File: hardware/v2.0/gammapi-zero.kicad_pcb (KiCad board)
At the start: 4 copper layers, 65 x 30 mm, 209 parts, among them IC1 IS42S16160J-6BLI, IC3 LM4040AIM3-2.0_NOPB, IC4 LTC2622IMS8#PBF, IC5 LTC6409IUDB#TRPBF, IC6 ADS6122IRHBT, J1 Conn_02x20_Counter_Clockwise, J2 GPDI_C_1.3, J3 USB_C_Receptacle_USB2.0_14P, J4 USB_C_Receptacle_USB2.0_14P, J5 USB_C_Receptacle_USB2.0_14P, J6 Micro_SD_Card_Det2, J7 RSP-122811-01, J8 BM04B-ACHSS-A-GAN-TF_LF__SN_, SW1 SW_Push, SW2 SW_Push, U1 ECP5U-25F-CABGA256, U10 TPD2EUSB30A, U12 W25Q128JVS, U2 LTC3407AEDD-2_PBF, U3 TLV62569DBV, U5 TCR5FM18A, U6 PCA9306DC1, U7 TPD2EUSB30A, U8 TPD2EUSB30A, U9 FT231XQ, Y1 SG-8018CG 50.000000MHz, Y2 SG-8018CG 50.000000MHz

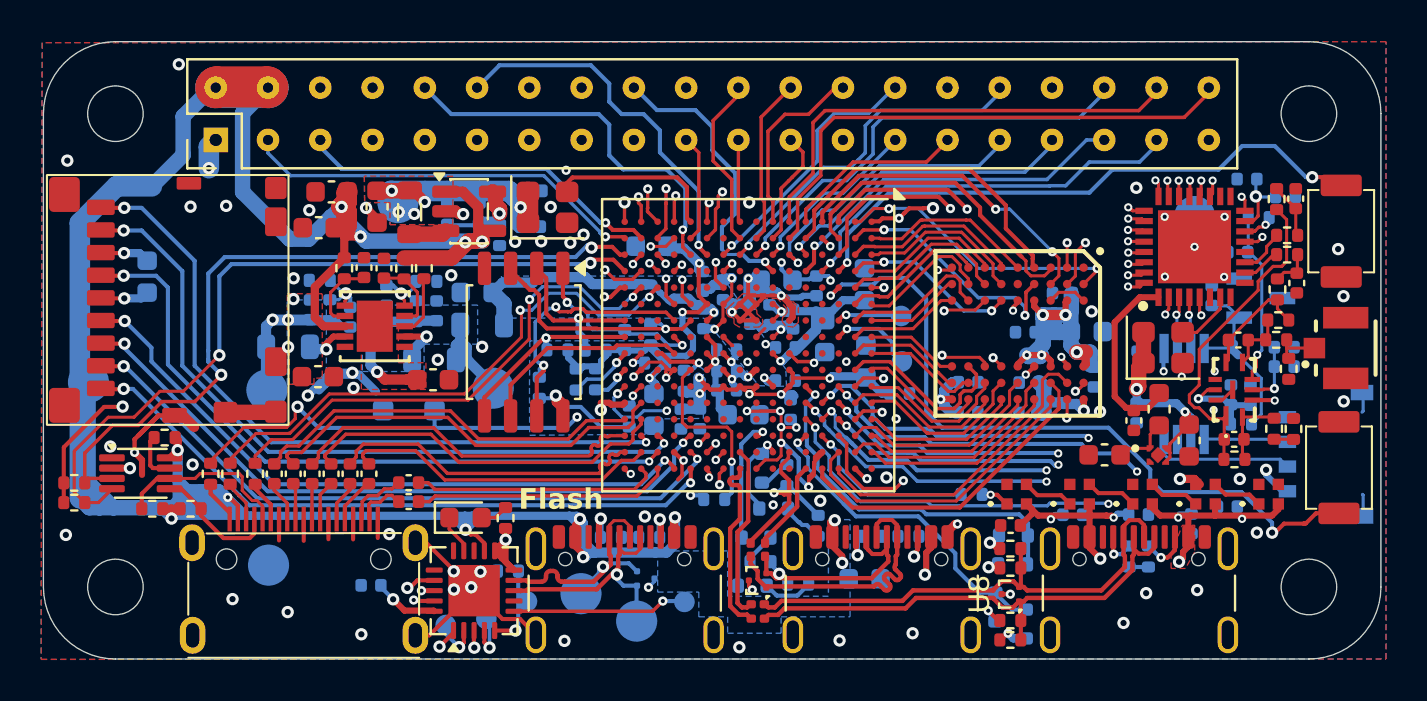
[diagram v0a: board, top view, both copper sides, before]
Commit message: Layout fixes
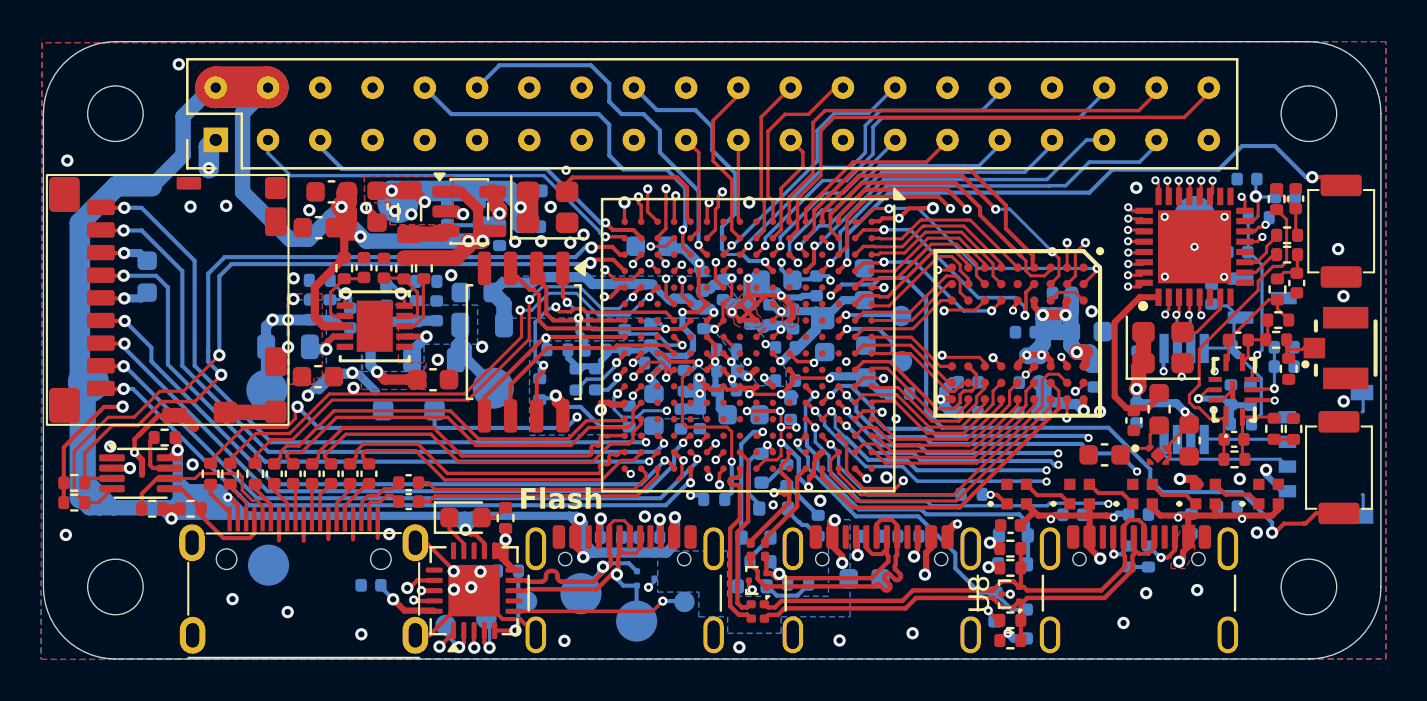
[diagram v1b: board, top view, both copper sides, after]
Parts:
- moved R47 0.07 mm to (139.9, 106.9)
- moved C83 0.07 mm to (172.5, 102.3)
- moved IC3 0.07 mm to (175.0, 102.5)

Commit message: Layout adjustments
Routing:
- net +3V3: track 144.3 -> 143.7 mm
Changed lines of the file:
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@@
 	)
 	(segment
-		(start 144.97153 108.71153)
-		(end 145.351296 108.71153)
+		(start 144.400001 107.760001)
+		(end 145.351296 108.711296)
 		(width 0.2)
 		(layer "In2.Cu")
@@
 	)
 	(segment
-		(start 146.125 117.65)
-		(end 146.044024 117.65)
+		(start 149.775 115.782247)
+		(end 148.891247 116.666)
 		(width 0.2)
 		(layer "In2.Cu")
@@
 	)
 	(segment
-		(start 137.204322 118.909)
-		(end 136.46591 118.909)
+		(start 137.402589 118.907411)
+		(end 137.205911 118.907411)
 		(width 0.2)
 		(layer "In2.Cu")
@@
 	)
 	(segment
-		(start 144.400001 107.209964)
-		(end 144.400001 108.140001)
+		(start 145.351296 108.71153)
+		(end 145.380765 108.741)
 		(width 0.2)
 		(layer "In2.Cu")
@@
 	)
 	(segment
-		(start 141.316 116.941)
-		(end 138.435667 116.941)
+		(start 148.618024 109.059)
+		(end 148.891 109.331976)
 		(width 0.2)
 		(layer "In2.Cu")
@@
 	)
 	(segment
-		(start 145.367171 117.65)
-		(end 142.025 117.65)
+		(start 145.351296 108.711296)
+		(end 145.351296 108.71153)
 		(width 0.2)
 		(layer "In2.Cu")
@@
 	)
 	(segment
-		(start 145.351296 108.71153)
-		(end 145.380765 108.741)
+		(start 146.044024 117.65)
+		(end 146.043024 117.651)
 		(width 0.2)
 		(layer "In2.Cu")
@@
 	)
 	(segment
-		(start 147.109 116.666)
-		(end 146.125 117.65)
+		(start 138.435667 116.941)
+		(end 137.61 117.766667)
 		(width 0.2)
 		(layer "In2.Cu")
@@
 	)
 	(segment
-		(start 144.399147 107.20911)
-		(end 144.400001 107.209964)
+		(start 141.316 116.941)
+		(end 138.435667 116.941)
 		(width 0.2)
 		(layer "In2.Cu")
@@
 	)
 	(segment
-		(start 136.46591 118.909)
-		(end 136.149 119.22591)
+		(start 137.204322 118.909)
+		(end 136.46591 118.909)
 		(width 0.2)
 		(layer "In2.Cu")
@@
 	)
 	(segment
-		(start 146.044024 117.65)
-		(end 146.043024 117.651)
+		(start 137.61 118.7)
+		(end 137.402589 118.907411)
+		(width 0.2)
+		(layer "In2.Cu")
+		(net 2)
+	)
+	(segment
+		(start 148.891 109.341)
+		(end 149.775 110.225)
 		(width 0.2)
 		(layer "In2.Cu")
@@
 	)
 	(segment
-		(start 145.380765 108.741)
-		(end 148.291 108.741)
+		(start 136.149 119.22591)
+		(end 136.149 119.227667)
 		(width 0.2)
 		(layer "In2.Cu")
@@
 	)
 	(segment
-		(start 148.618024 109.059)
-		(end 148.891 109.331976)
+		(start 146.125 117.65)
+		(end 146.044024 117.65)
 		(width 0.2)
 		(layer "In2.Cu")
@@
 	)
 	(segment
-		(start 149.775 110.225)
-		(end 149.775 115.782247)
-		(width 0.2)
-		(layer "In2.Cu")
-		(net 2)
-	)
-	(segment
-		(start 148.891 109.331976)
-		(end 148.891 109.341)
+		(start 148.891247 116.666)
+		(end 147.109 116.666)
 		(width 0.2)
 		(layer "In2.Cu")
@@
 	)
 	(segment
-		(start 149.775 115.782247)
-		(end 148.891247 116.666)
+		(start 137.61 117.766667)
+		(end 137.61 118.7)
 		(width 0.2)
 		(layer "In2.Cu")
@@
 	)
 	(segment
-		(start 137.61 118.7)
-		(end 137.402589 118.907411)
+		(start 137.205911 118.907411)
+		(end 137.204322 118.909)
 		(width 0.2)
 		(layer "In2.Cu")
@@
 	)
 	(segment
-		(start 148.891 109.341)
-		(end 149.775 110.225)
+		(start 148.291 108.741)
+		(end 148.609 109.059)
 		(width 0.2)
 		(layer "In2.Cu")
@@
 	)
 	(segment
-		(start 148.291 108.741)
-		(end 148.609 109.059)
+		(start 147.109 116.666)
+		(end 146.125 117.65)
 		(width 0.2)
 		(layer "In2.Cu")
@@
 	)
 	(segment
-		(start 138.435667 116.941)
-		(end 137.61 117.766667)
+		(start 136.149 119.227667)
+		(end 135.950381 119.426286)
 		(width 0.2)
 		(layer "In2.Cu")
@@
 	)
 	(segment
-		(start 144.400001 108.140001)
-		(end 144.97153 108.71153)
+		(start 145.380765 108.741)
+		(end 148.291 108.741)
 		(width 0.2)
 		(layer "In2.Cu")
@@
 	)
 	(segment
-		(start 137.402589 118.907411)
-		(end 137.205911 118.907411)
+		(start 148.891 109.331976)
+		(end 148.891 109.341)
 		(width 0.2)
 		(layer "In2.Cu")
@@
 	)
 	(segment
-		(start 137.61 117.766667)
-		(end 137.61 118.7)
+		(start 142.025 117.65)
+		(end 141.316 116.941)
 		(width 0.2)
 		(layer "In2.Cu")
@@
 	)
 	(segment
-		(start 136.149 119.22591)
-		(end 136.149 119.227667)
+		(start 136.46591 118.909)
+		(end 136.149 119.22591)
 		(width 0.2)
 		(layer "In2.Cu")
@@
 	)
 	(segment
-		(start 136.149 119.227667)
-		(end 135.950381 119.426286)
+		(start 149.775 110.225)
+		(end 149.775 115.782247)
 		(width 0.2)
 		(layer "In2.Cu")
@@
 	)
 	(segment
-		(start 148.891247 116.666)
-		(end 147.109 116.666)
+		(start 144.399147 107.20911)
+		(end 144.400001 107.209964)
 		(width 0.2)
 		(layer "In2.Cu")
@@
 	)
 	(segment
-		(start 142.025 117.65)
-		(end 141.316 116.941)
+		(start 145.367171 117.65)
+		(end 142.025 117.65)
 		(width 0.2)
 		(layer "In2.Cu")
@@
 	)
 	(segment
-		(start 137.205911 118.907411)
-		(end 137.204322 118.909)
+		(start 144.400001 107.209964)
+		(end 144.400001 107.760001)
 		(width 0.2)
 		(layer "In2.Cu")
@@
 	)
 	(segment
-		(start 147.15399 112)
-		(end 147.025 112)
-		(width 0.2)
-		(layer "In2.Cu")
-		(net 18)
-	)
-	(segment
 		(start 147.303631 102.715329)
 		(end 148.792358 102.715329)
@@
 	)
 	(segment
-		(start 147.025 112)
-		(end 146.675 111.65)
-		(width 0.2)
-		(layer "In2.Cu")
-		(net 18)
-	)
-	(segment
 		(start 148.792358 102.715329)
 		(end 149.213999 103.13697)
@@
 	)
 	(segment
+		(start 146.23 104.52)
+		(end 146.56 104.19)
+		(width 0.3)
+		(layer "In2.Cu")
+		(net 54)
+	)
+	(segment
 		(start 128.243999 103.32)
 		(end 128.237999 103.326)
@@
 	)
 	(segment
-		(start 141.685 108.24214)
-		(end 142.04214 108.24214)
-		(width 0.15)
-		(layer "In2.Cu")
-		(net 88)
-	)
-	(segment
-		(start 142.857 109.057)
-		(end 144.825596 109.057)
-		(width 0.15)
-		(layer "In2.Cu")
-		(net 88)
-	)
-	(segment
-		(start 147.107 109.057)
-		(end 147.571233 109.521233)
+		(start 142.04214 108.24214)
+		(end 142.82753 109.02753)
 		(width 0.15)
 		(layer "In2.Cu")
@@
 	)
 	(segment
-		(start 142.04214 108.24214)
-		(end 142.857 109.057)
+		(start 145.249874 109.057)
+		(end 147.107 109.057)
 		(width 0.15)
 		(layer "In2.Cu")
@@
 	)
 	(segment
-		(start 145.249874 109.057)
-		(end 147.107 109.057)
+		(start 141.685 108.24214)
+		(end 142.04214 108.24214)
 		(width 0.15)
 		(layer "In2.Cu")
@@
 	)
 	(segment
-		(start 144.825596 109.057)
-		(end 144.855066 109.02753)
+		(start 147.107 109.057)
+		(end 147.571233 109.521233)
 		(width 0.15)
 		(layer "In2.Cu")
@@
 	)
 	(segment
-		(start 144.855066 109.02753)
+		(start 142.82753 109.02753)
 		(end 145.220404 109.02753)
 		(width 0.15)
@@
 	)
 	(segment
-		(start 161.9 105.36)
-		(end 161.9 105.448617)
+		(start 158.28 107.65)
+		(end 156.870868 107.65)
 		(width 0.15)
 		(layer "In2.Cu")
@@
 	)
 	(segment
-		(start 156.510869 108.010001)
-		(end 156.510868 108.01)
+		(start 161.078617 106.27)
+		(end 159.66 106.27)
 		(width 0.15)
 		(layer "In2.Cu")
@@
 	)
 	(segment
-		(start 161.228617 106.12)
-		(end 159.9 106.12)
+		(start 161.9 105.448617)
+		(end 161.078617 106.27)
 		(width 0.15)
 		(layer "In2.Cu")
@@
 	)
 	(segment
-		(start 156.872255 108.010001)
-		(end 156.510869 108.010001)
+		(start 161.9 105.36)
+		(end 161.9 105.448617)
 		(width 0.15)
 		(layer "In2.Cu")
@@
 	)
 	(segment
-		(start 161.9 105.448617)
-		(end 161.228617 106.12)
+		(start 156.510869 108.010001)
+		(end 156.510868 108.01)
 		(width 0.15)
 		(layer "In2.Cu")
@@
 	)
 	(segment
-		(start 158.17 107.85)
-		(end 157.032256 107.85)
+		(start 159.66 106.27)
+		(end 158.28 107.65)
 		(width 0.15)
 		(layer "In2.Cu")
@@
 	)
 	(segment
-		(start 159.9 106.12)
-		(end 158.17 107.85)
+		(start 156.870868 107.65)
+		(end 156.510869 108.009999)
 		(width 0.15)
 		(layer "In2.Cu")
@@
 	)
 	(segment
-		(start 157.032256 107.85)
-		(end 156.872255 108.010001)
+		(start 156.510869 108.009999)
+		(end 156.510869 108.010001)
 		(width 0.15)
 		(layer "In2.Cu")
@@
 		(polygon
 			(pts
-				(xy 149 112) (xy 149 120) (xy 115.65 120) (xy 115.66 112)
+				(xy 146.16 112.01) (xy 146.87 112.57) (xy 146.87 120.01) (xy 115.65 120) (xy 115.66 112)
 			)
 		)
